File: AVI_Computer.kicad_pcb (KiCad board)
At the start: 2 copper layers, 14 parts, among them IC1 ESP32-S2-MINI-2U-N4, IC2 LM3671MF-3.3_NOPB, IC3 LM3671MF-3.3_NOPB, IC4 BMP390, IC5 BMI270, J1 USB4105-GF-A-060

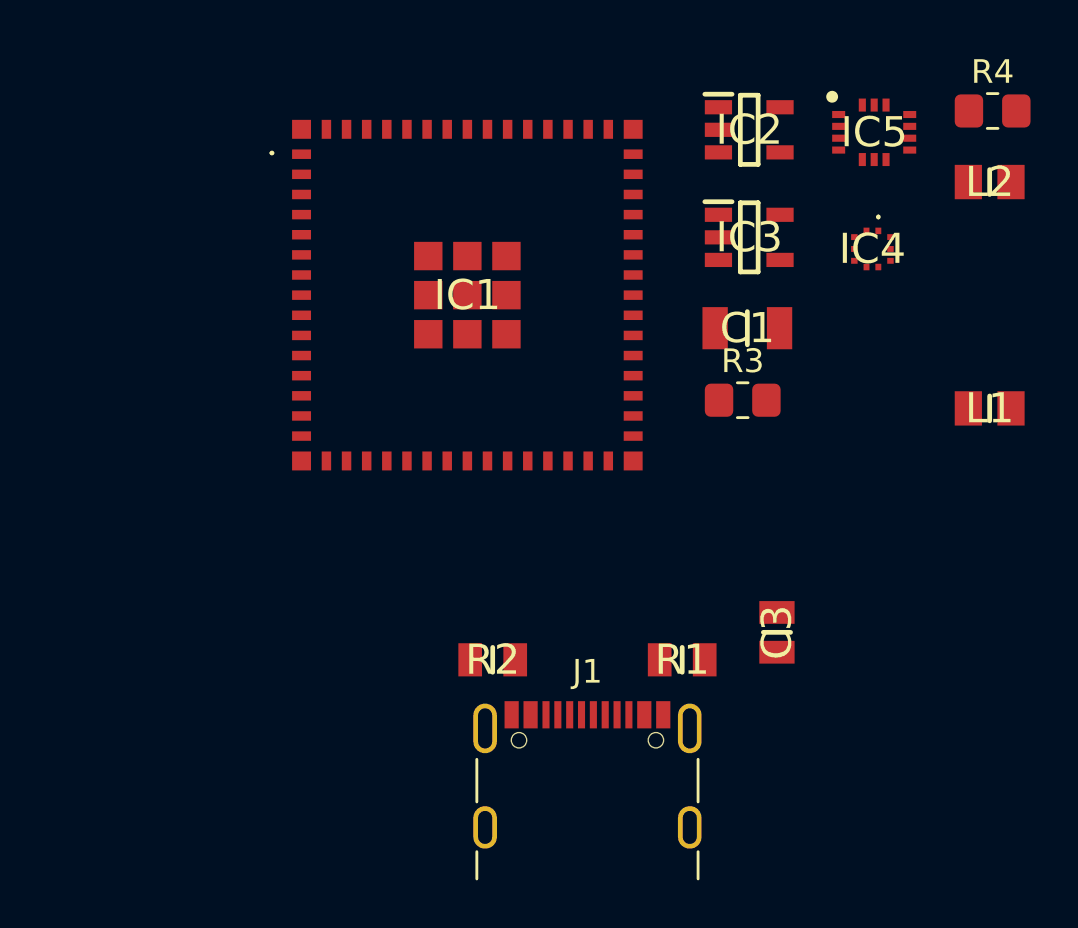
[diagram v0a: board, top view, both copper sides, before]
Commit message: cghanges
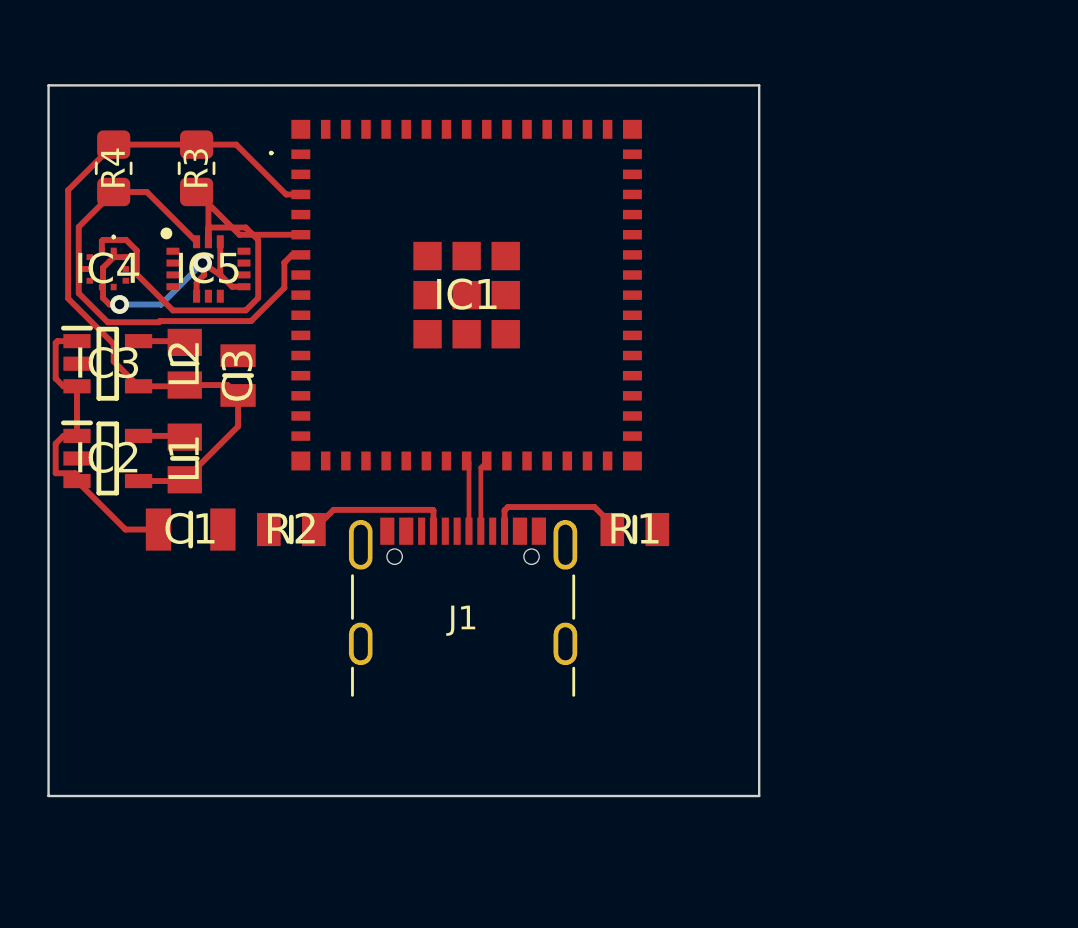
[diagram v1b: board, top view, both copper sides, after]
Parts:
- moved R4 37.2 mm to (146.0, 105.2), turned to 90 degrees
- moved L2 34.8 mm to (149.0, 113.5), turned to -90 degrees
- moved L1 34.0 mm to (149.0, 117.5), turned to -90 degrees
- moved IC4 32.3 mm to (145.8, 109.5)
- moved IC2 30.4 mm to (145.8, 117.5)
- moved IC5 28.7 mm to (150.0, 109.5)
- moved IC3 27.6 mm to (145.8, 113.5)
- moved C3 25.2 mm to (151.2, 114.0), turned to 90 degrees
- moved R3 25.0 mm to (149.5, 105.2), turned to 90 degrees
- moved C1 25.0 mm to (149.2, 120.5)
- moved R2 10.1 mm to (153.5, 120.5)
- moved J1 9.36 mm to (160.8, 124.2)
- moved R1 5.85 mm to (168.0, 120.5)
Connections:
- IC1 pad 5: unconnected-(IC1-IO1-Pad5) -> /scl
- IC1 pad 6: unconnected-(IC1-IO2-Pad6) -> /sda
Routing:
- net /3v3: track 0.00 -> 45.0 mm, vias 0 -> 2
- net /scl: track 0.00 -> 21.9 mm
- net /sda: track 0.00 -> 21.4 mm
- net +5V: track 0.00 -> 13.3 mm
- net Net-(J1-CC1): track 0.00 -> 6.28 mm
- net Net-(J1-CC2): track 0.00 -> 6.00 mm
- net /D+: track 0.00 -> 3.08 mm
- net /D-: track 0.00 -> 2.99 mm
- net Net-(IC3-SW): track 0.00 -> 1.97 mm
- net Net-(IC2-SW): track 0.00 -> 1.97 mm
- added copper zone on F.Cu, net GND
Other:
- board outline added: 30 x 30 mm
